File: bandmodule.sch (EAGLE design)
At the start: 15 parts

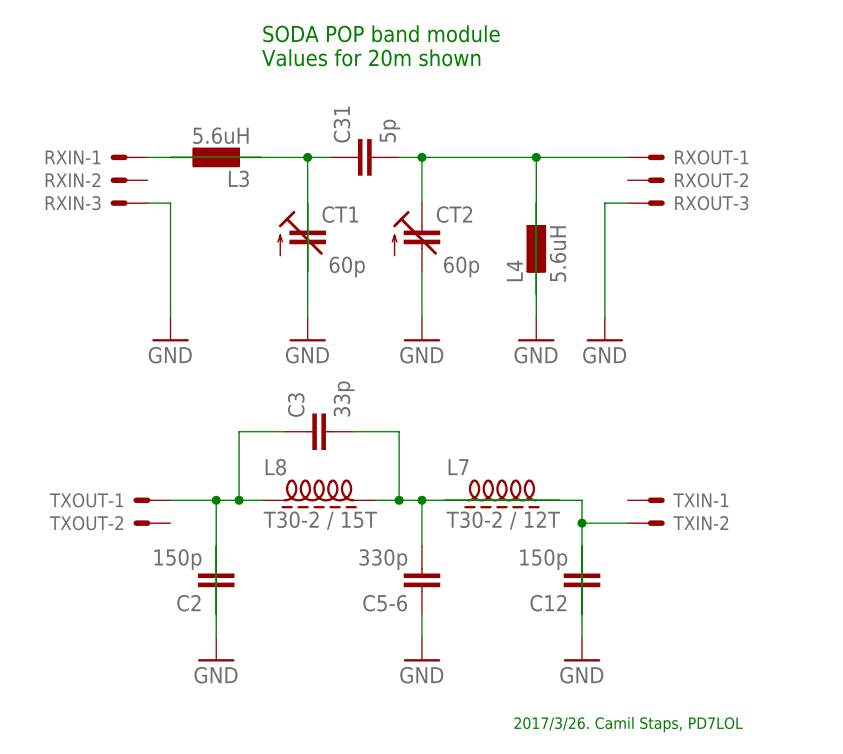
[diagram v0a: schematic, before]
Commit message: Readme, made more space for toroids
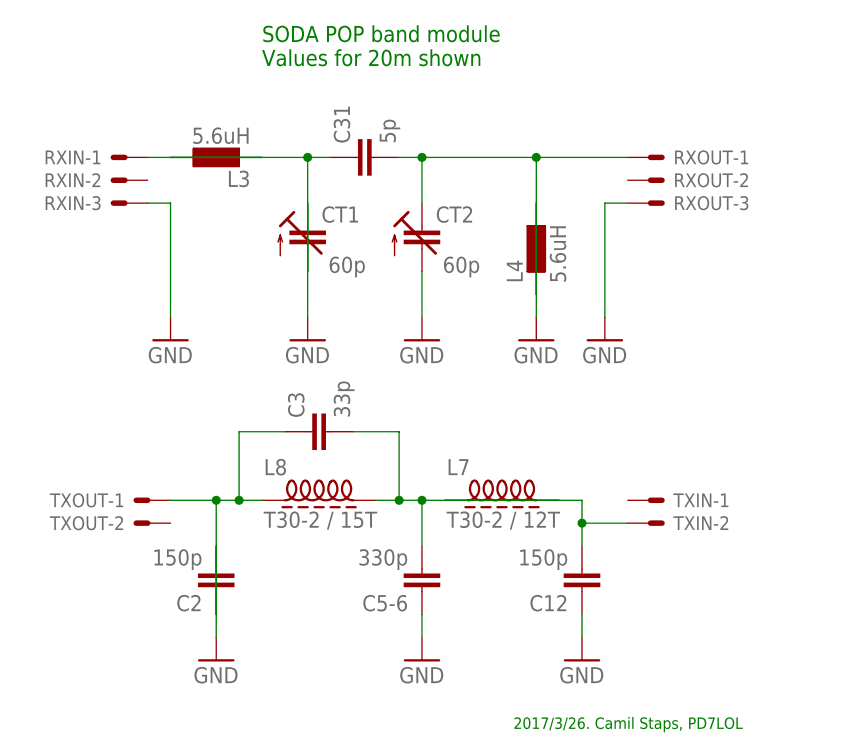
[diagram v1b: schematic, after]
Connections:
- net GND: now also C12.1; no longer C12.2
- net N$6: now also C12.2; no longer C12.1
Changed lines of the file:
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@@
 </segment>
 <segment>
-<pinref part="C12" gate="G$1" pin="2"/>
+<pinref part="C12" gate="G$1" pin="1"/>
 <pinref part="GND8" gate="1" pin="GND"/>
-<wire x1="66.04" y1="22.86" x2="66.04" y2="12.7" width="0.1524" layer="91"/>
+<wire x1="66.04" y1="15.24" x2="66.04" y2="12.7" width="0.1524" layer="91"/>
 </segment>
 </net>
@@
 <segment>
 <pinref part="L7" gate="G$1" pin="1"/>
-<pinref part="C12" gate="G$1" pin="1"/>
+<pinref part="C12" gate="G$1" pin="2"/>
 <wire x1="50.8" y1="27.94" x2="66.04" y2="27.94" width="0.1524" layer="91"/>
 <wire x1="66.04" y1="27.94" x2="66.04" y2="25.4" width="0.1524" layer="91"/>
 <pinref part="TXIN" gate="-2" pin="S"/>
-<wire x1="66.04" y1="25.4" x2="66.04" y2="15.24" width="0.1524" layer="91"/>
+<wire x1="66.04" y1="25.4" x2="66.04" y2="22.86" width="0.1524" layer="91"/>
 <wire x1="66.04" y1="25.4" x2="71.12" y2="25.4" width="0.1524" layer="91"/>
 <junction x="66.04" y="25.4"/>
